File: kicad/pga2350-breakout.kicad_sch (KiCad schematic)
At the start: 10 parts, among them J1 Conn_01x02_Pin, J10 Conn_02x05_Counter_Clockwise, J2 Conn_02x05_Odd_Even, J3 Conn_01x02_Pin, J4 Conn_01x05_Pin, J5 Conn_02x05_Counter_Clockwise, J6 Conn_02x05_Counter_Clockwise, J7 Conn_02x05_Counter_Clockwise, J8 Conn_02x05_Counter_Clockwise

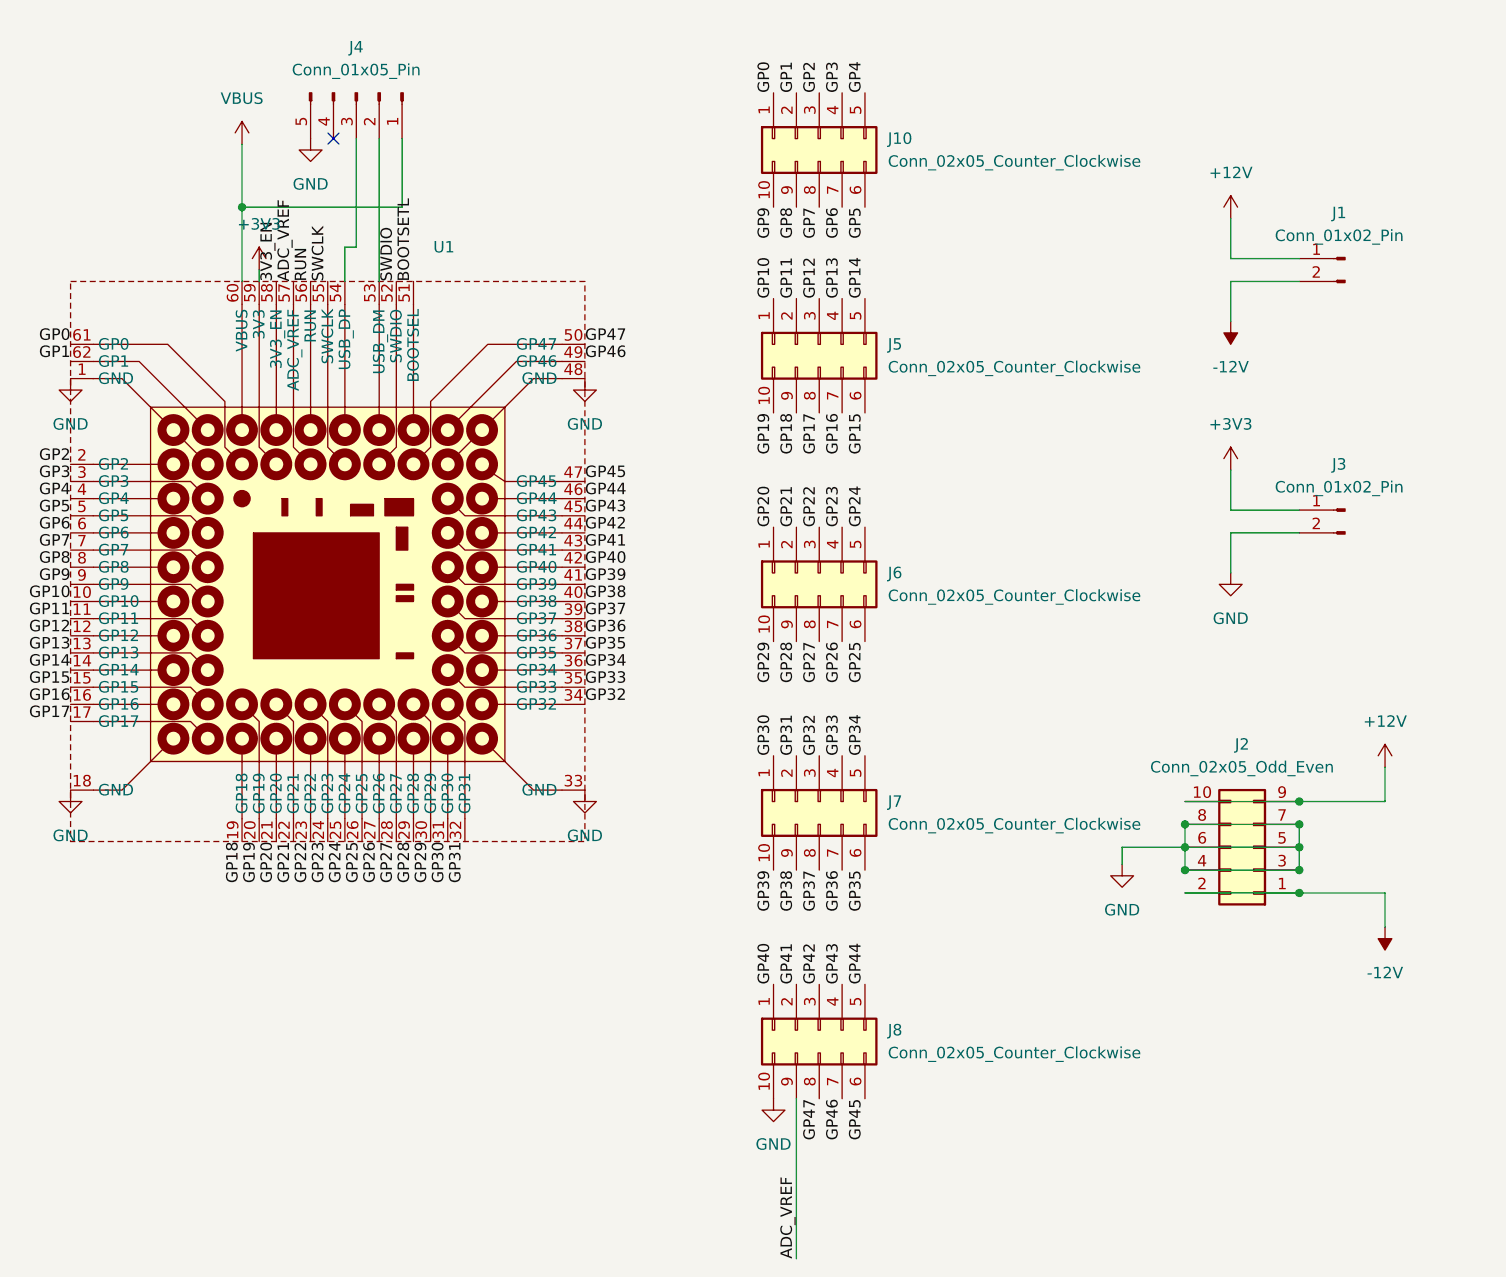
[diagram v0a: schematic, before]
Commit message: save production version 1.0
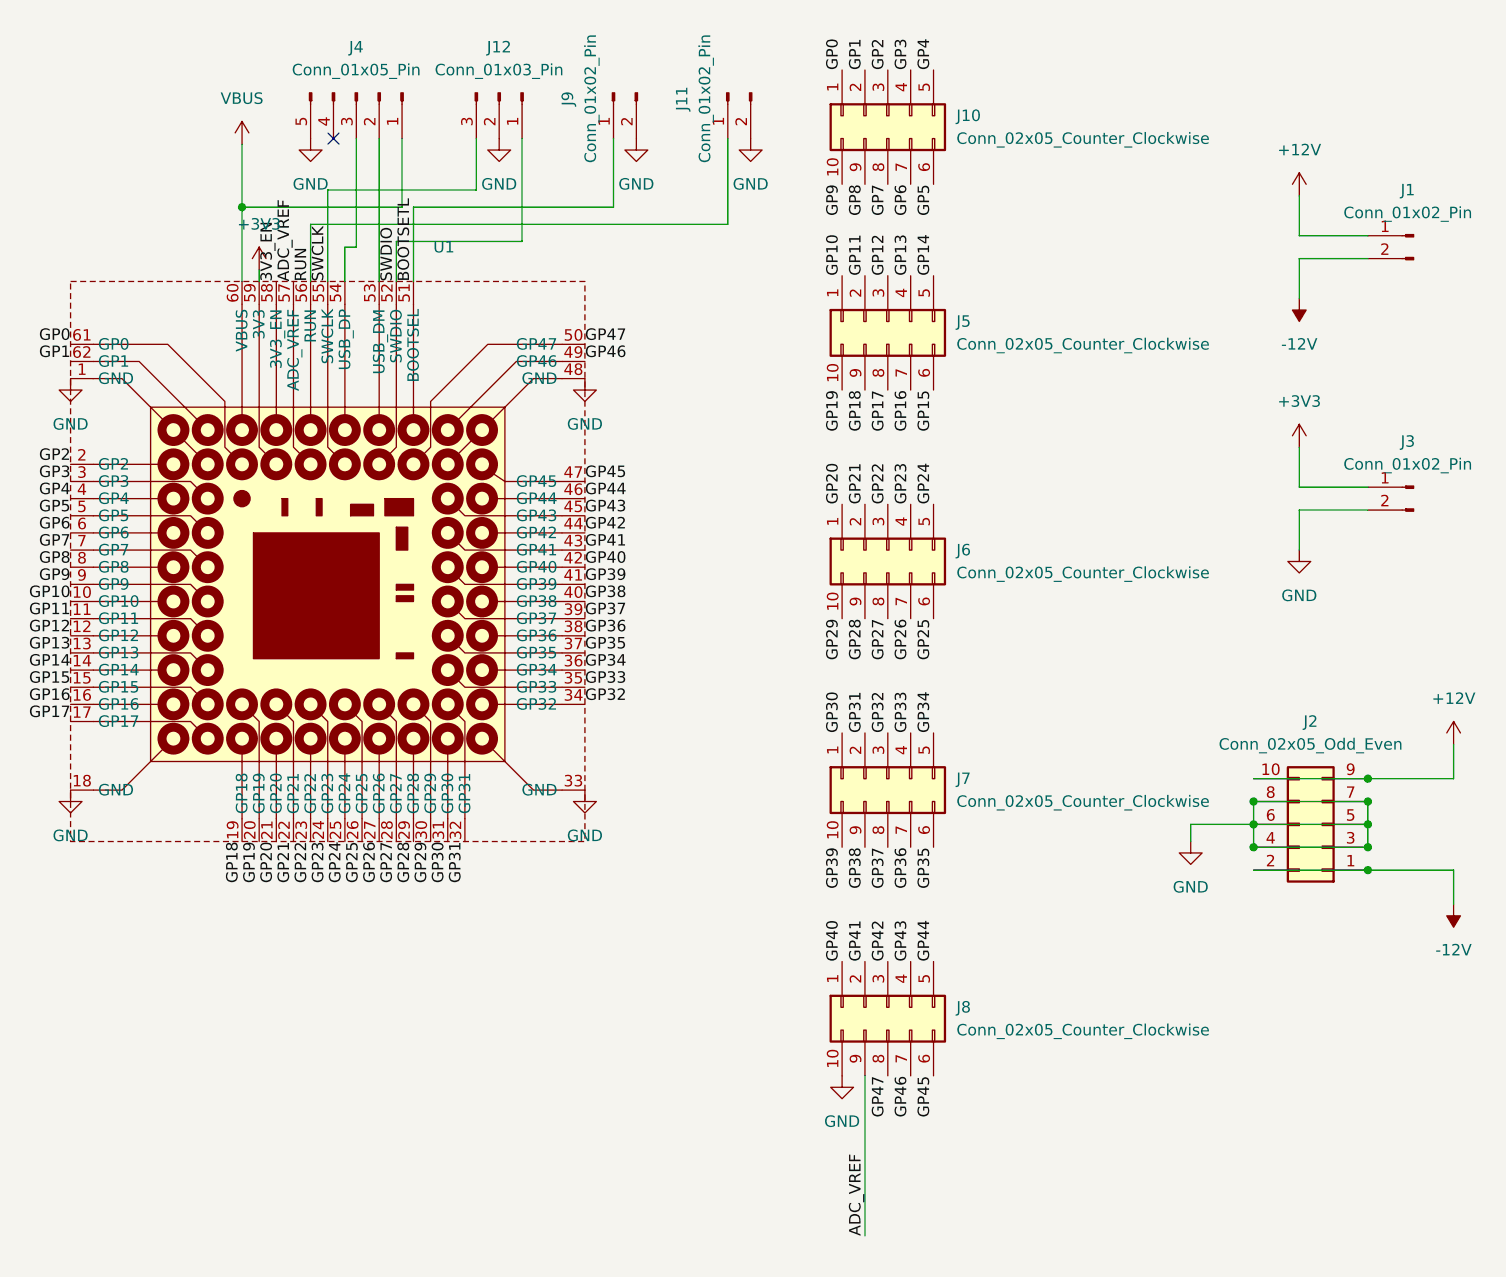
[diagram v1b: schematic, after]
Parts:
- added J11, J9: Conn_01x02_Pin, allen-synthesis:pin-socket-2.54mm-01x02, symbol Connector:Conn_01x02_Pin
- added J12: Conn_01x03_Pin, allen-synthesis:pin-header-2.54mm-01x03, symbol Connector:Conn_01x03_Pin
- J1, J3: footprint Connector_PinSocket_2.54mm:PinSocket_1x02_P2.54mm_Vertical -> allen-synthesis:pin-socket-2.54mm-01x02
- J10, J5, J6, J7, J8: footprint Connector_PinSocket_2.54mm:PinSocket_2x05_P2.54mm_Vertical -> allen-synthesis:pin-socket-2.54mm-02x05
- J4: footprint Connector_PinHeader_2.54mm:PinHeader_1x05_P2.54mm_Vertical -> allen-synthesis:pin-header-2.54mm-01x05
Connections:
- net BOOTSETL: now also J9.1 (Pin_1)
- net GND: now also J11.2 (Pin_2), J12.2 (Pin_2), J9.2 (Pin_2)
- net RUN: now also J11.1 (Pin_1)
- net SWCLK: now also J12.3 (Pin_3)
- net SWDIO: now also J12.1 (Pin_1)
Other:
- moved on the sheet: J1, J10, J2, J3, J5, J6, J7, J8
